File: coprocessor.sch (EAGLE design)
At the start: 32 parts, among them IC1 MEGA32U2, J1 AVR_SPI_PRG_6NS

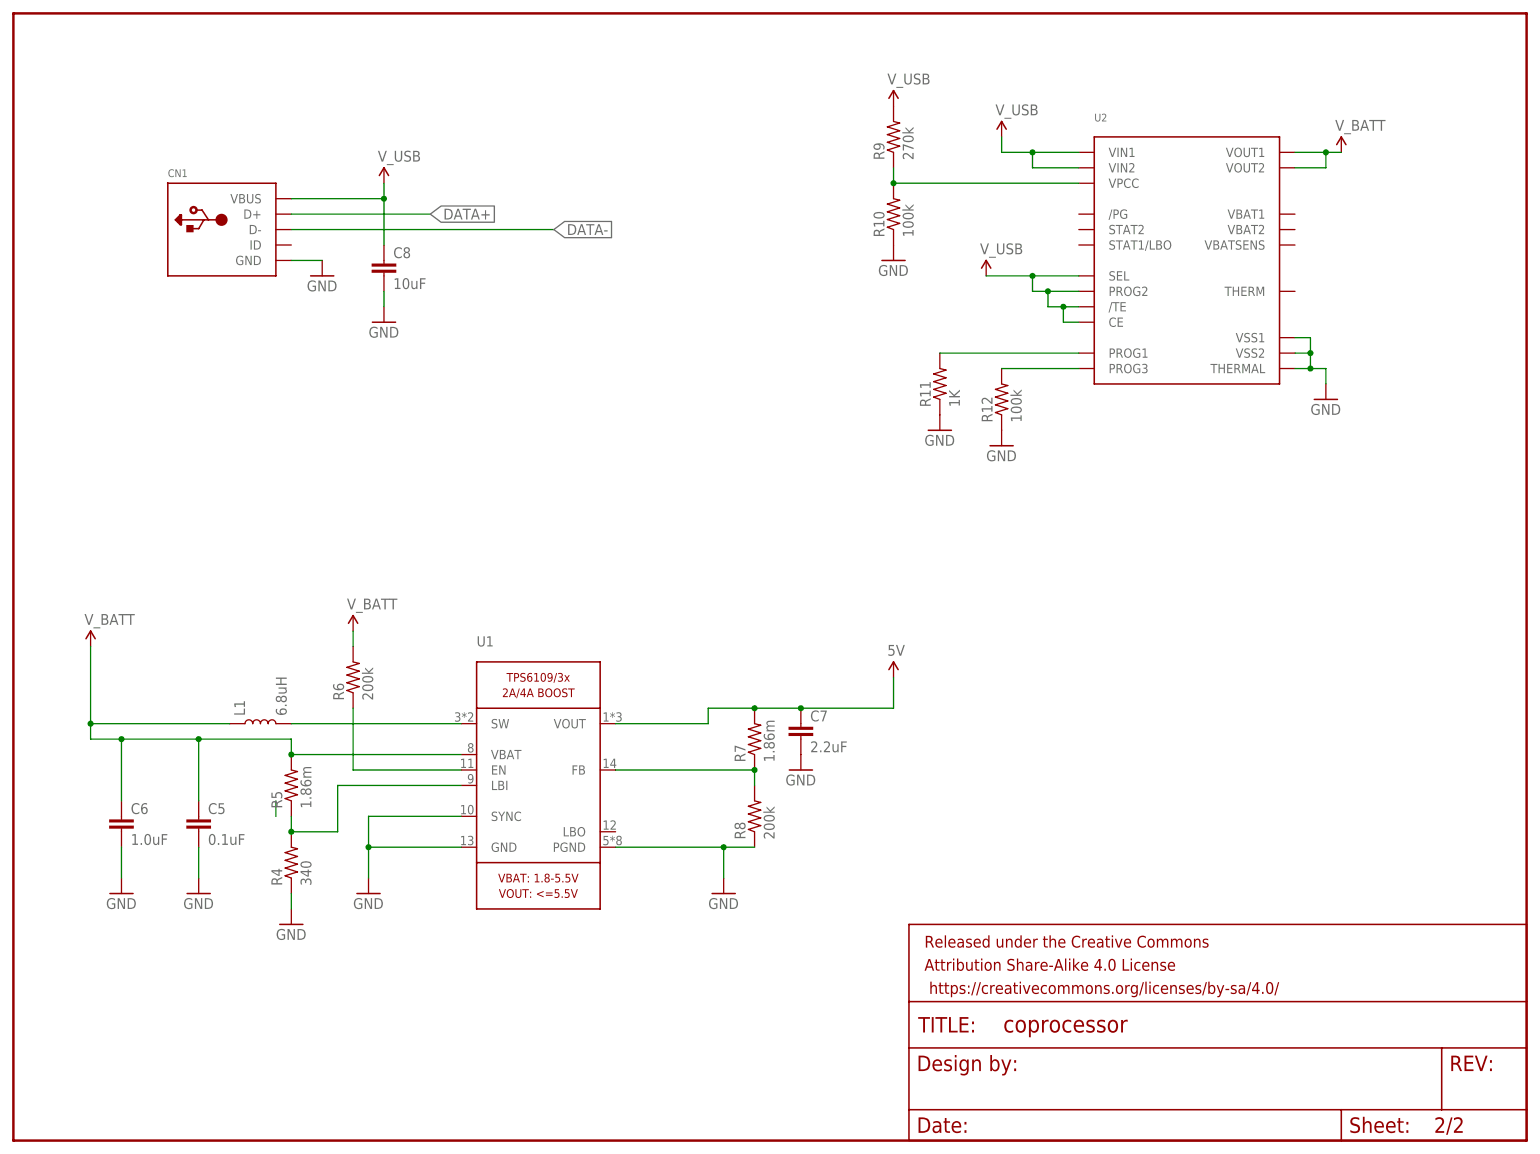
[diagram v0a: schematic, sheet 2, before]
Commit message: finished the power
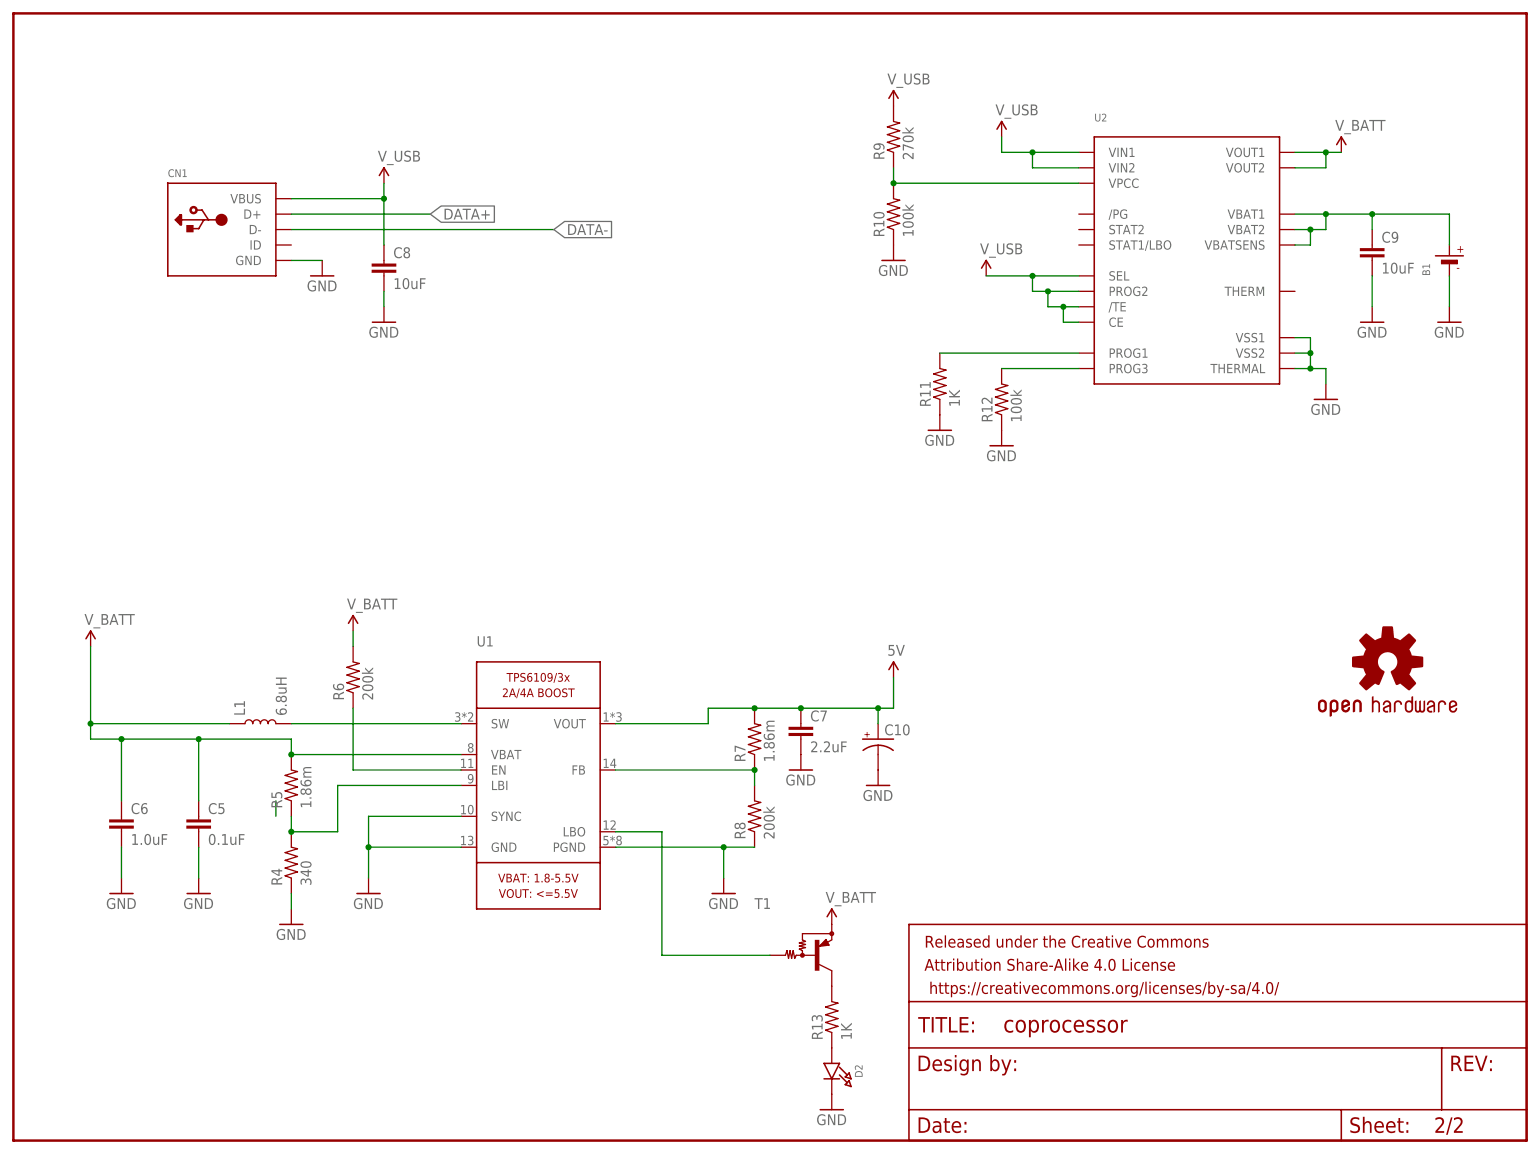
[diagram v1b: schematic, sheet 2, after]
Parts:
- added B1: (no value), custom:MICROBUILDER_BATTERY
- added C10: (no value), SparkFun-Capacitors:CAP_POL1206
- added C9: 10uF, SparkFun-Capacitors:10UF-6.3V-20%(0603)
- added D2: (no value), custom:MICROBUILDER_LED0603
- added LOGO1: OSHW-LOGOS, SparkFun-Aesthetics:OSHW-LOGOS
- added R13: 1K, SparkFun-Resistors:1KOHM-1/10W-1%(0603)
- added T1: (no value), custom:TRANSISTOR_PNP_DRIVERMUN2111T1SC59-BEC
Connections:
- new net N$15: T1.B, U1.LBO
- new net N$16: R13.2, T1.C
- new net N$17: D2.A, R13.1
- new net N$8: B1.+, C9.1, U2.VBAT1, U2.VBAT2, U2.VBATSENS
- net 5V: now also C10.+
- net GND: now also B1.-, C10.-, C9.2, D2.C
- net V_BATT: now also T1.E
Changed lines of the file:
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@@
 <part name="GND21" library="SparkFun-Aesthetics" deviceset="GND" device=""/>
 <part name="SUPPLY14" library="SparkFun-Aesthetics" deviceset="V_BATT" device=""/>
+<part name="B1" library="custom" deviceset="MICROBUILDER_BATTERY" device=""/>
+<part name="LOGO1" library="SparkFun-Aesthetics" deviceset="OSHW-LOGO" device="S"/>
+<part name="C9" library="SparkFun-Capacitors" deviceset="10UF-6.3V-20%(0603)" device="" value="10uF"/>
+<part name="GND22" library="SparkFun-Aesthetics" deviceset="GND" device=""/>
+<part name="GND23" library="SparkFun-Aesthetics" deviceset="GND" device=""/>
+<part name="T1" library="custom" deviceset="TRANSISTOR_PNP_DRIVER" device="SC59-BEC" technology="MUN2111T1"/>
+<part name="SUPPLY15" library="SparkFun-Aesthetics" deviceset="V_BATT" device=""/>
+<part name="R13" library="SparkFun-Resistors" deviceset="1KOHM-1/10W-1%(0603)" device="" value="1K"/>
+<part name="D2" library="custom" deviceset="MICROBUILDER_LED" device="0603"/>
+<part name="GND24" library="SparkFun-Aesthetics" deviceset="GND" device=""/>
+<part name="C10" library="SparkFun-Capacitors" deviceset="CAP_POL" device="1206"/>
+<part name="GND25" library="SparkFun-Aesthetics" deviceset="GND" device=""/>
 </parts>
 <sheets>
@@
 <instance part="GND21" gate="1" x="256.54" y="137.16"/>
 <instance part="SUPPLY14" gate="G$1" x="259.08" y="177.8"/>
+<instance part="B1" gate="G$1" x="276.86" y="160.02" rot="R90"/>
+<instance part="LOGO1" gate="G$1" x="266.7" y="93.98"/>
+<instance part="C9" gate="G$1" x="264.16" y="160.02"/>
+<instance part="GND22" gate="1" x="264.16" y="149.86"/>
+<instance part="GND23" gate="1" x="276.86" y="149.86"/>
+<instance part="T1" gate="G$1" x="172.72" y="45.72"/>
+<instance part="SUPPLY15" gate="G$1" x="175.26" y="50.8"/>
+<instance part="R13" gate="G$1" x="175.26" y="35.56" rot="R90"/>
+<instance part="D2" gate="G$1" x="175.26" y="25.4" rot="R270"/>
+<instance part="GND24" gate="1" x="175.26" y="20.32"/>
+<instance part="C10" gate="G$1" x="182.88" y="81.28"/>
+<instance part="GND25" gate="1" x="182.88" y="73.66"/>
 </instances>
 <busses>
@@
 <wire x1="254" y1="147.32" x2="254" y2="144.78" width="0.1524" layer="91"/>
 <junction x="254" y="144.78"/>
+</segment>
+<segment>
+<pinref part="C9" gate="G$1" pin="2"/>
+<pinref part="GND22" gate="1" pin="GND"/>
+<wire x1="264.16" y1="157.48" x2="264.16" y2="152.4" width="0.1524" layer="91"/>
+</segment>
+<segment>
+<pinref part="B1" gate="G$1" pin="-"/>
+<pinref part="GND23" gate="1" pin="GND"/>
+<wire x1="276.86" y1="157.48" x2="276.86" y2="152.4" width="0.1524" layer="91"/>
+</segment>
+<segment>
+<pinref part="D2" gate="G$1" pin="C"/>
+<pinref part="GND24" gate="1" pin="GND"/>
+</segment>
+<segment>
+<pinref part="C10" gate="G$1" pin="-"/>
+<pinref part="GND25" gate="1" pin="GND"/>
 </segment>
 </net>
@@
 <junction x="256.54" y="177.8"/>
 </segment>
+<segment>
+<pinref part="T1" gate="G$1" pin="E"/>
+<pinref part="SUPPLY15" gate="G$1" pin="V_BATT"/>
+</segment>
 </net>
 <net name="N$11" class="0">
@@
 <pinref part="SUPPLY10" gate="G$1" pin="5V"/>
 <wire x1="162.56" y1="86.36" x2="170.18" y2="86.36" width="0.1524" layer="91"/>
-<wire x1="170.18" y1="86.36" x2="185.42" y2="86.36" width="0.1524" layer="91"/>
+<wire x1="170.18" y1="86.36" x2="182.88" y2="86.36" width="0.1524" layer="91"/>
+<wire x1="182.88" y1="86.36" x2="185.42" y2="86.36" width="0.1524" layer="91"/>
 <wire x1="185.42" y1="86.36" x2="185.42" y2="91.44" width="0.1524" layer="91"/>
 <pinref part="R7" gate="G$1" pin="2"/>
@@
 <wire x1="154.94" y1="86.36" x2="162.56" y2="86.36" width="0.1524" layer="91"/>
 <junction x="162.56" y="86.36"/>
+<pinref part="C10" gate="G$1" pin="+"/>
+<wire x1="182.88" y1="83.82" x2="182.88" y2="86.36" width="0.1524" layer="91"/>
+<junction x="182.88" y="86.36"/>
 </segment>
 </net>
@@
 </segment>
 </net>
+<net name="N$8" class="0">
+<segment>
+<pinref part="U2" gate="G$1" pin="VBAT1"/>
+<pinref part="B1" gate="G$1" pin="+"/>
+<wire x1="251.46" y1="167.64" x2="256.54" y2="167.64" width="0.1524" layer="91"/>
+<wire x1="256.54" y1="167.64" x2="264.16" y2="167.64" width="0.1524" layer="91"/>
+<wire x1="264.16" y1="167.64" x2="276.86" y2="167.64" width="0.1524" layer="91"/>
+<wire x1="276.86" y1="167.64" x2="276.86" y2="162.56" width="0.1524" layer="91"/>
+<pinref part="C9" gate="G$1" pin="1"/>
+<wire x1="264.16" y1="165.1" x2="264.16" y2="167.64" width="0.1524" layer="91"/>
+<junction x="264.16" y="167.64"/>
+<pinref part="U2" gate="G$1" pin="VBAT2"/>
+<wire x1="251.46" y1="165.1" x2="254" y2="165.1" width="0.1524" layer="91"/>
+<wire x1="254" y1="165.1" x2="256.54" y2="165.1" width="0.1524" layer="91"/>
+<wire x1="256.54" y1="165.1" x2="256.54" y2="167.64" width="0.1524" layer="91"/>
+<junction x="256.54" y="167.64"/>
+<pinref part="U2" gate="G$1" pin="VBATSENS"/>
+<wire x1="251.46" y1="162.56" x2="254" y2="162.56" width="0.1524" layer="91"/>
+<wire x1="254" y1="162.56" x2="254" y2="165.1" width="0.1524" layer="91"/>
+<junction x="254" y="165.1"/>
+</segment>
+</net>
+<net name="N$15" class="0">
+<segment>
+<pinref part="U1" gate="G$1" pin="LBO"/>
+<wire x1="139.7" y1="66.04" x2="147.32" y2="66.04" width="0.1524" layer="91"/>
+<wire x1="147.32" y1="66.04" x2="147.32" y2="45.72" width="0.1524" layer="91"/>
+<wire x1="147.32" y1="45.72" x2="165.1" y2="45.72" width="0.1524" layer="91"/>
+<pinref part="T1" gate="G$1" pin="B"/>
+</segment>
+</net>
+<net name="N$16" class="0">
+<segment>
+<pinref part="T1" gate="G$1" pin="C"/>
+<pinref part="R13" gate="G$1" pin="2"/>
+</segment>
+</net>
+<net name="N$17" class="0">
+<segment>
+<pinref part="R13" gate="G$1" pin="1"/>
+<pinref part="D2" gate="G$1" pin="A"/>
+</segment>
+</net>
